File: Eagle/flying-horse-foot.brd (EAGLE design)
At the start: 55.8 x 32.5 mm, 20 parts, among them U1 8U2-AU, Y1 16MHz

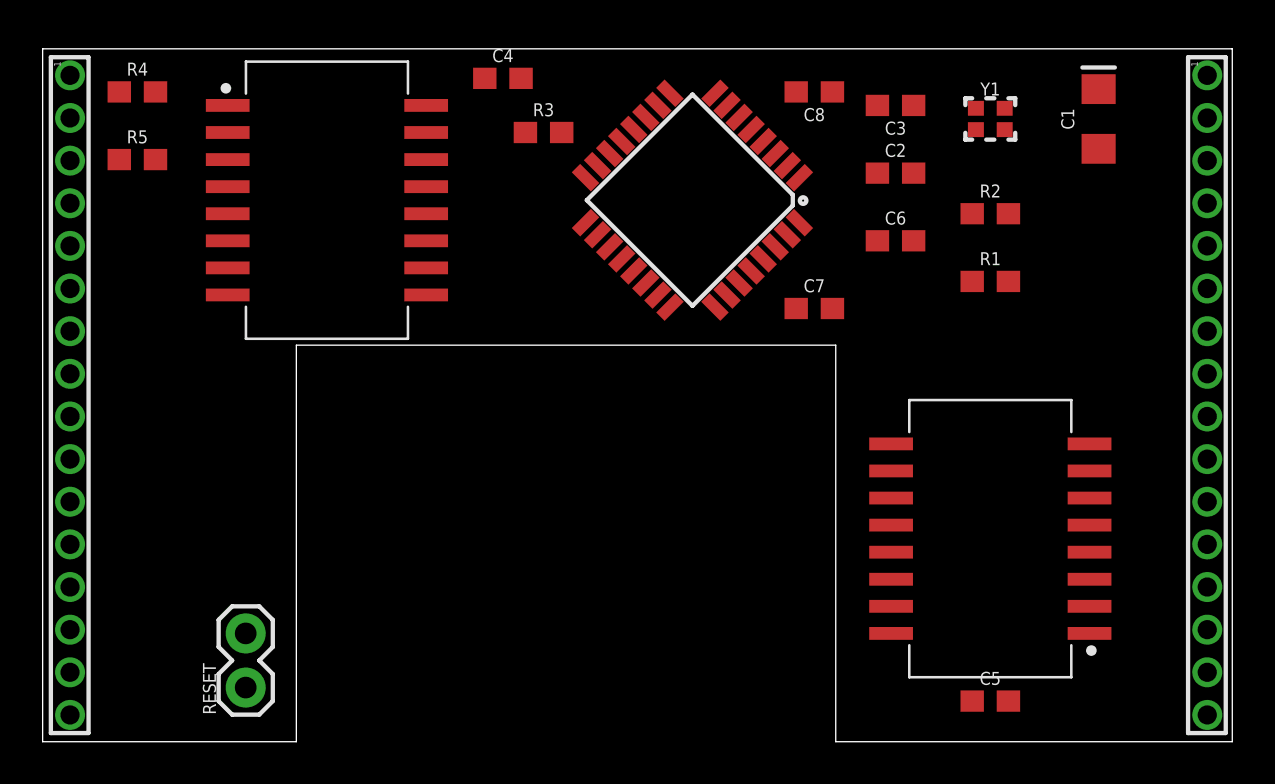
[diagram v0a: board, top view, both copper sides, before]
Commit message: rel 1
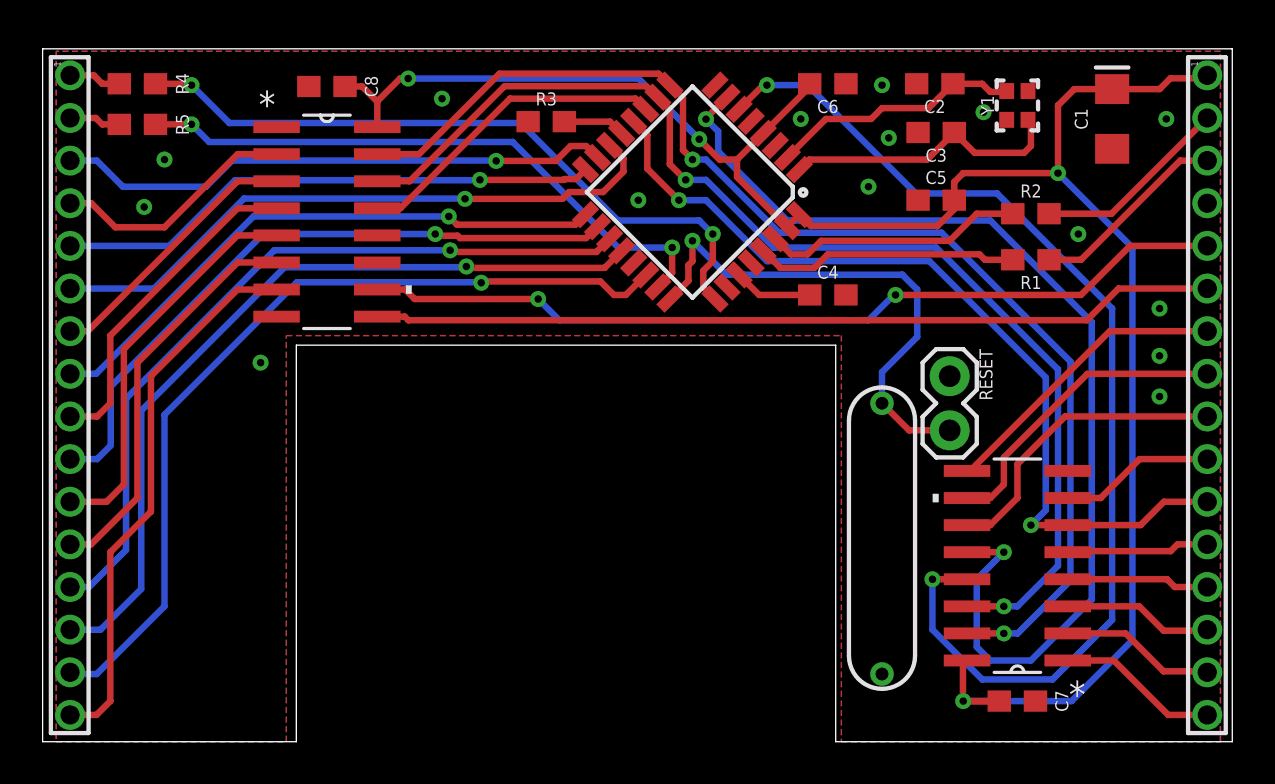
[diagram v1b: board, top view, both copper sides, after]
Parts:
- added S1: MK6-5-B, switch-reed:MK6-5
- C4, C6: value 0.1uF -> 1.0uF
- C7, C8: value 1.0uF -> 0.1uF
- U$1, U$2: value 74HC42 -> 74HC42D16; device aaa2:SOIC127P1032X265-16N -> aaa2:D16
- moved RESET 36.1 mm to (42.5, 17.1), turned to 270 degrees
- moved C5 23.6 mm to (41.9, 25.4)
- moved C8 22.9 mm to (13.3, 30.7)
- moved C7 20.7 mm to (45.7, 1.91)
- moved C4 18.3 mm to (36.8, 21.0)
- moved C6 8.02 mm to (36.8, 30.9), turned to 180 degrees
- moved C2 4.58 mm to (41.8, 30.9), turned to 180 degrees
- moved C3 2.29 mm to (41.9, 28.6)
- moved R1 2.16 mm to (46.4, 22.6)
- moved R2 1.90 mm to (46.4, 24.8)
- moved U$1 1.80 mm to (45.7, 8.26)
- moved R5 1.65 mm to (4.45, 29.0)
- moved Y1 1.42 mm to (45.7, 29.8), turned to 90 degrees
- moved U$2 1.02 mm to (13.3, 24.4)
- moved C1 0.63 mm to (50.2, 29.2)
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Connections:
- removed net N$9: RESET.2, U1.24
- new net RESET: RESET.2, S1.1, U1.24
- net COL-3: no longer U$4.13
- net COL-5: now also U$4.13
- net GND: now also C5.1, C8.2, S1.2; no longer C5.2, C8.1
- net N$3: now also C2.1; no longer C3.1
- net N$4: now also C3.1; no longer C2.1
- net N$6: now also C4.1; no longer C7.1
- net VCC: now also C5.2, C7.1, C8.1; no longer C4.1, C5.1, C8.2
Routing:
- net VCC: track 0.00 -> 94.5 mm, vias 0 -> 4
- net ROW-A: track 0.00 -> 57.2 mm, vias 0 -> 2
- net ROW-B: track 0.00 -> 55.1 mm, vias 0 -> 2
- net ROW-C: track 0.00 -> 51.5 mm, vias 0 -> 2
- net ROW-D: track 0.00 -> 50.6 mm, vias 0 -> 2
- net ROW-5: track 0.00 -> 41.2 mm, vias 0 -> 2
- net ROW-18: track 0.00 -> 41.0 mm, vias 0 -> 2
- net COL-12: track 0.00 -> 40.6 mm, vias 0 -> 1
- net ROW-17: track 0.00 -> 39.6 mm
- net COL-6: track 0.00 -> 38.2 mm, vias 0 -> 1
- net COL-5: track 0.00 -> 36.3 mm, vias 0 -> 1
- net N$5: track 0.00 -> 32.5 mm, vias 0 -> 2
- net COL-4: track 0.00 -> 31.1 mm, vias 0 -> 1
- net COL-0: track 0.00 -> 29.8 mm, vias 0 -> 1
- net N$7: track 0.00 -> 28.7 mm, vias 0 -> 2
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- added copper zone on layer 1, net GND
- added copper zone on layer 16, net GND
